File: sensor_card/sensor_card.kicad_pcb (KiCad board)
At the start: 2 copper layers, 72.4 x 86 mm, 18 parts, among them J1 Raspberry_Pi_4, J10 Conn_01x05, J2 BME280, J3 GPS, J4 PARACHUTE, J5 Conn_01x02, J6 power LORA, J7 power_RPI, J8 MPU_6500, U1 Ai-Thinker-Ra-02

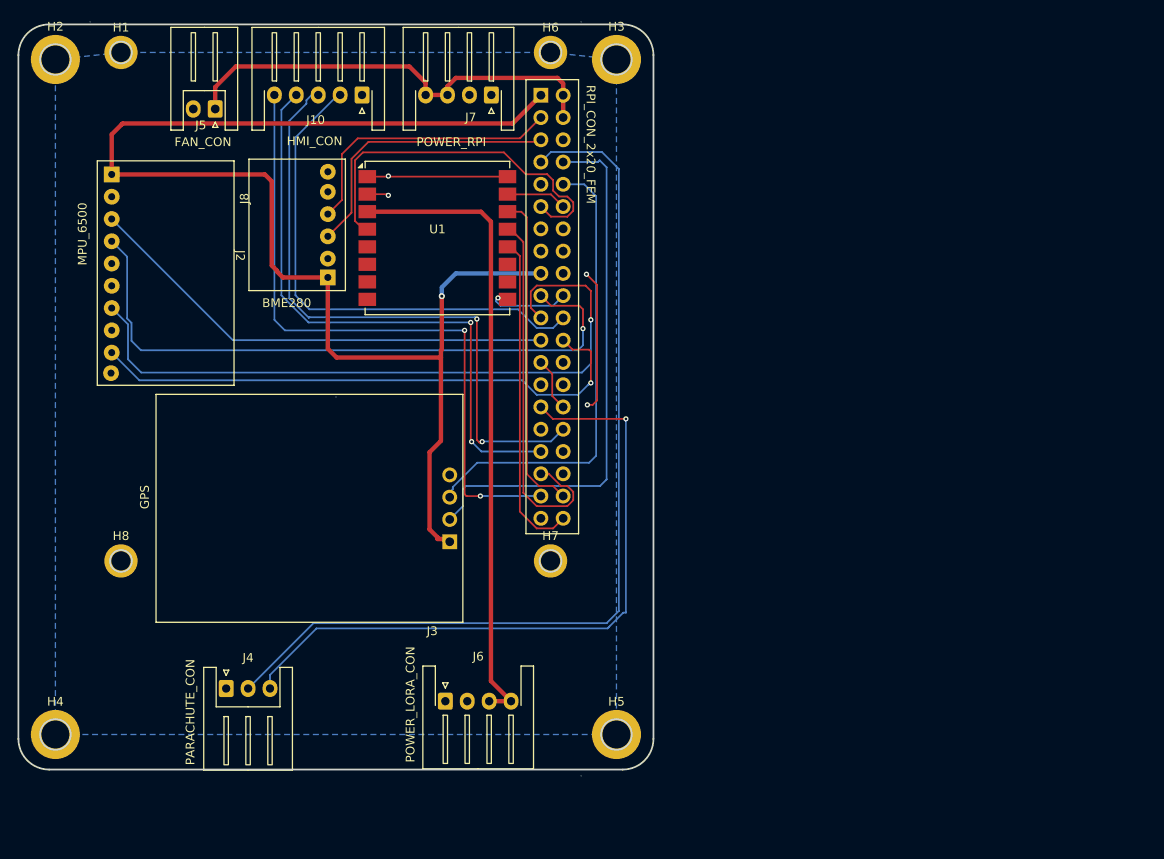
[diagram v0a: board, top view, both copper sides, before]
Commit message: sensor card: full revision
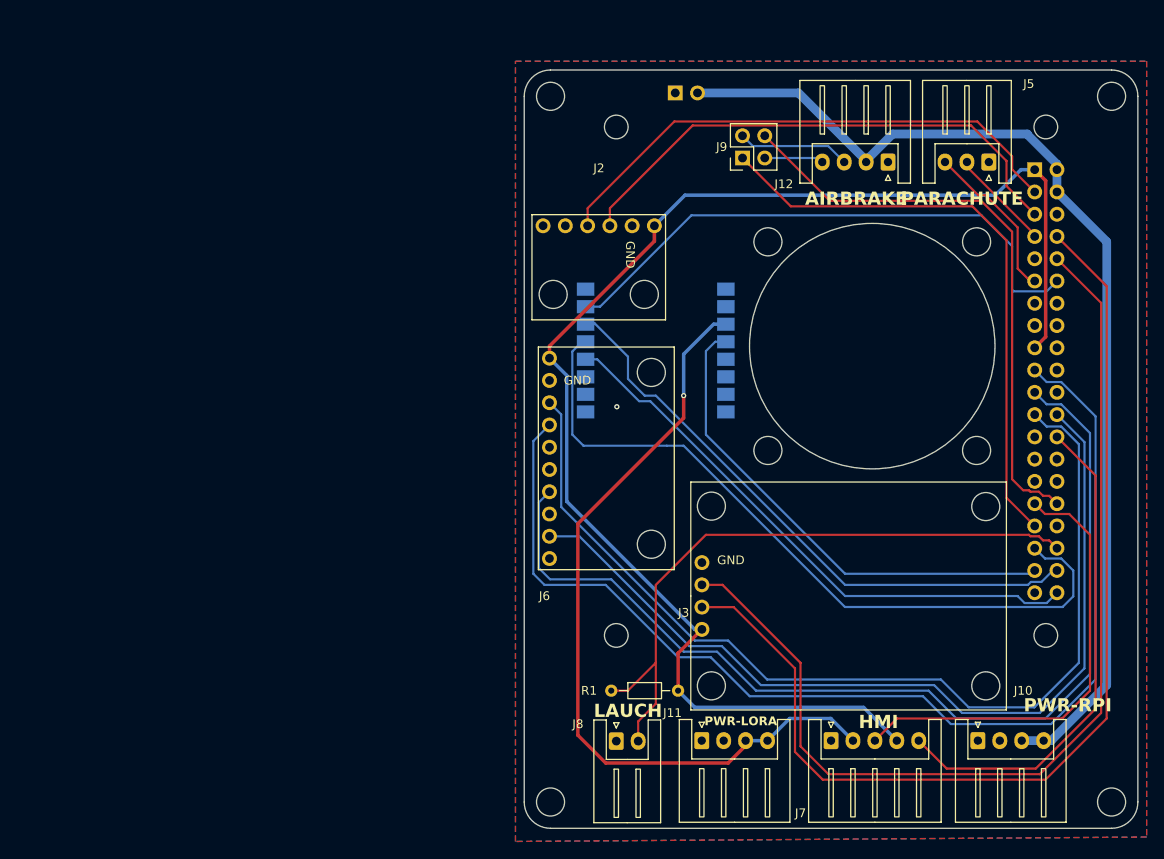
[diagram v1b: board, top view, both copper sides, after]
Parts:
- added J11: power LORA, Connector_JST:JST_XH_S4B-XH-A_1x04_P2.50mm_Horizontal, F.Cu at (148.8, 120.0)
- added J12: AIRBRAKE, Connector_JST:JST_XH_S4B-XH-A_1x04_P2.50mm_Horizontal, F.Cu at (170.0, 54.0)
- added J9: proto_selector, Connector_PinHeader_2.54mm:PinHeader_2x02_P2.54mm_Vertical, F.Cu at (153.4, 53.5)
- added R1: 10k, Resistor_THT:R_Axial_DIN0204_L3.6mm_D1.6mm_P7.62mm_Horizontal, F.Cu at (138.4, 114.3)
- H1: value MountingHole_RPI -> MountingHole_3.2mm_M3; footprint MountingHole:MountingHole_2.2mm_M2_DIN965_Pad -> MountingHole:MountingHole_3.2mm_M3
- H2, H3, H4: value MountingHole_Pad -> MountingHole_3.2mm_M3; footprint MountingHole:MountingHole_3.2mm_M3_DIN965_Pad -> MountingHole:MountingHole_3.2mm_M3
- H5: value MountingHole_Pad -> MountingHole_2.7mm_M2.5; footprint MountingHole:MountingHole_3.2mm_M3_DIN965_Pad -> MountingHole:MountingHole_2.7mm_M2.5
- H6, H7, H8: value MountingHole_RPI -> MountingHole_2.7mm_M2.5; footprint MountingHole:MountingHole_2.2mm_M2_DIN965_Pad -> MountingHole:MountingHole_2.7mm_M2.5
- J1: value Raspberry_Pi_4 -> fan_power; footprint Connector_PinSocket_2.54mm:PinSocket_2x20_P2.54mm_Vertical -> Connector_PinHeader_2.54mm:PinHeader_1x02_P2.54mm_Horizontal
- J10: value Conn_01x05 -> power_RPI; footprint Connector_JST:JST_XH_S5B-XH-A-1_1x05_P2.50mm_Horizontal -> Connector_JST:JST_XH_S4B-XH-A_1x04_P2.50mm_Horizontal
- J2: value BME280 -> BME; footprint PHOENIX:BME 280 -> nasa:BME280
- J3: footprint PHOENIX:GPS-MV2 -> nasa:GPS
- J4: value PARACHUTE -> Raspberry_Pi_4; footprint Connector_JST:JST_XH_S3B-XH-A_1x03_P2.50mm_Horizontal -> Connector_PinSocket_2.54mm:PinSocket_2x20_P2.54mm_Vertical; moved to B.Cu
- J5: value Conn_01x02 -> PARACHUTE; footprint Connector_JST:JST_XH_S2B-XH-A_1x02_P2.50mm_Horizontal -> Connector_JST:JST_XH_S3B-XH-A_1x03_P2.50mm_Horizontal
- J6: value power LORA -> MPU_6500; footprint Connector_JST:JST_XH_S4B-XH-A-1_1x04_P2.50mm_Horizontal -> nasa:MPU6500
- J7: value power_RPI -> hmi; footprint Connector_JST:JST_XH_S4B-XH-A-1_1x04_P2.50mm_Horizontal -> Connector_JST:JST_XH_S5B-XH-A_1x05_P2.50mm_Horizontal
- J8: value MPU_6500 -> lauch; footprint PHOENIX:MPU-9250 -> Connector_JST:JST_XH_S2B-XH-A_1x02_P2.50mm_Horizontal
- U1: moved to B.Cu
- moved H4 120.7 mm to (195.5, 127.0)
- moved H2 120.6 mm to (195.5, 46.5)
- moved J4 109.6 mm to (186.7, 54.9), turned to 180 degrees
- moved H8 105.8 mm to (188.0, 108.0)
- moved J10 101.8 mm to (180.2, 120.0), turned to 0 degrees
- moved J5 88.5 mm to (181.5, 54.0)
- moved H3 85.0 mm to (131.5, 127.0)
- moved J7 83.2 mm to (163.5, 120.0), turned to 0 degrees
- moved J8 74.5 mm to (139.0, 120.1), turned to 0 degrees
- moved H5 69.3 mm to (139.0, 50.0)
- moved H6 57.1 mm to (188.0, 50.0)
- moved H1 49.3 mm to (131.5, 46.5)
- moved J3 40.0 mm to (142.7, 103.5), turned to 90 degrees
- moved J2 35.1 mm to (137.0, 55.2), turned to 0 degrees
- moved J6 28.5 mm to (126.3, 87.8), turned to 90 degrees
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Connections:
- J1 pad 1: +3V3 -> GND
- J10 pad 2: /LED_ALIM_RPI_CAPTEURS -> GND
- J10 pad 3: /LED_ALIM_LORA -> +5V
- J10 pad 4: /LED_FONC_LORA -> +5V
- J2 pad 5: (no net) -> unconnected-(J2-Pin_5-Pad5)
- J2 pad 6: (no net) -> unconnected-(J2-Pin_6-Pad6)
- J3 pad 1: +3V3 -> GND
- J3 pad 2: /GPS_RX -> /GPS_TX
- J3 pad 3: /GPS_TX -> /GPS_RX
- J3 pad 4: GND -> +3V3
- J4 pad 1: GND -> +3V3
- J4 pad 2: /PARACHUTE_ACTIVATION -> +5V
- J4 pad 3: /PARA_STATE_FEEDBACK -> /SDA
- J5 pad 1: +5V -> GND
- J5 pad 2: GND -> /PARACHUTE_ACTIVATION
- J6 pad 1: GND -> +3V3
- J6 pad 3: +3V3_LORA -> /MPU_SCK
- J6 pad 4: +3V3_LORA -> /MPU_MOSI
- J7 pad 2: GND -> +3V3_LORA
- J7 pad 3: +5V -> /LED_LORA_WORKING
- J7 pad 4: +5V -> +3V3
- J8 pad 1: +3V3 -> GND
- J8 pad 2: GND -> /lauch_detect
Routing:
- net /PARACHUTE_ACTIVATION: track 106.6 -> 11.7 mm
- net /PARA_STATE_FEEDBACK: track 77.5 -> 0.00 mm, vias 1 -> 0
- net /LED_FONC_PROGRAMMES: track 75.3 -> 0.00 mm, vias 2 -> 0
- net /lauch_detect: track 0.00 -> 73.8 mm
- net /LED_ALIM_LORA: track 71.8 -> 0.00 mm, vias 2 -> 0
- net +5V: track 50.9 -> 121.4 mm
- net /LED_FONC_LORA: track 68.4 -> 0.00 mm, vias 2 -> 0
- net /AIRBRAKE_RX_SCL: track 0.00 -> 67.9 mm
- net /AIRBRAKE_TX_SDA: track 0.00 -> 67.2 mm
- net /GPS_TX: track 52.9 -> 116.9 mm
- net /MPU_SCK: track 54.7 -> 114.5 mm
- net /LORA_CS: track 6.93 -> 65.1 mm
- net /LED_ALIM_RPI_CAPTEURS: track 57.7 -> 0.00 mm
- net /GPS_RX: track 62.6 -> 120.1 mm
- net /LED_PROG_WORKING: track 0.00 -> 57.2 mm
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- added copper zone on F.Cu, net GND
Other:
- board size 72.4 x 86 mm -> 70 x 86.5 mm
- board text added: "AIRBRAKE"
- board text added: "GND"
- board text added: "HMI"
- board text added: "LAUCH"
- board text added: "PARACHUTE"
- board text added: "PWR-LORA"
- board text added: "PWR-RPI"
- board text removed: "BME280"
- board text removed: "FAN_CON"
- board text removed: "GPS"
- board text removed: "HMI_CON"
- board text removed: "LORA"
- board text removed: "MPU_6500"
- board text removed: "PARACHUTE_CON"
- board text removed: "POWER_LORA_CON"
- board text removed: "POWER_RPI"
- board text removed: "RPI_CON_2x20_FEM"
